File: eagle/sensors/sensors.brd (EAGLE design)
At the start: 51.7 x 35.5 mm, 4 parts

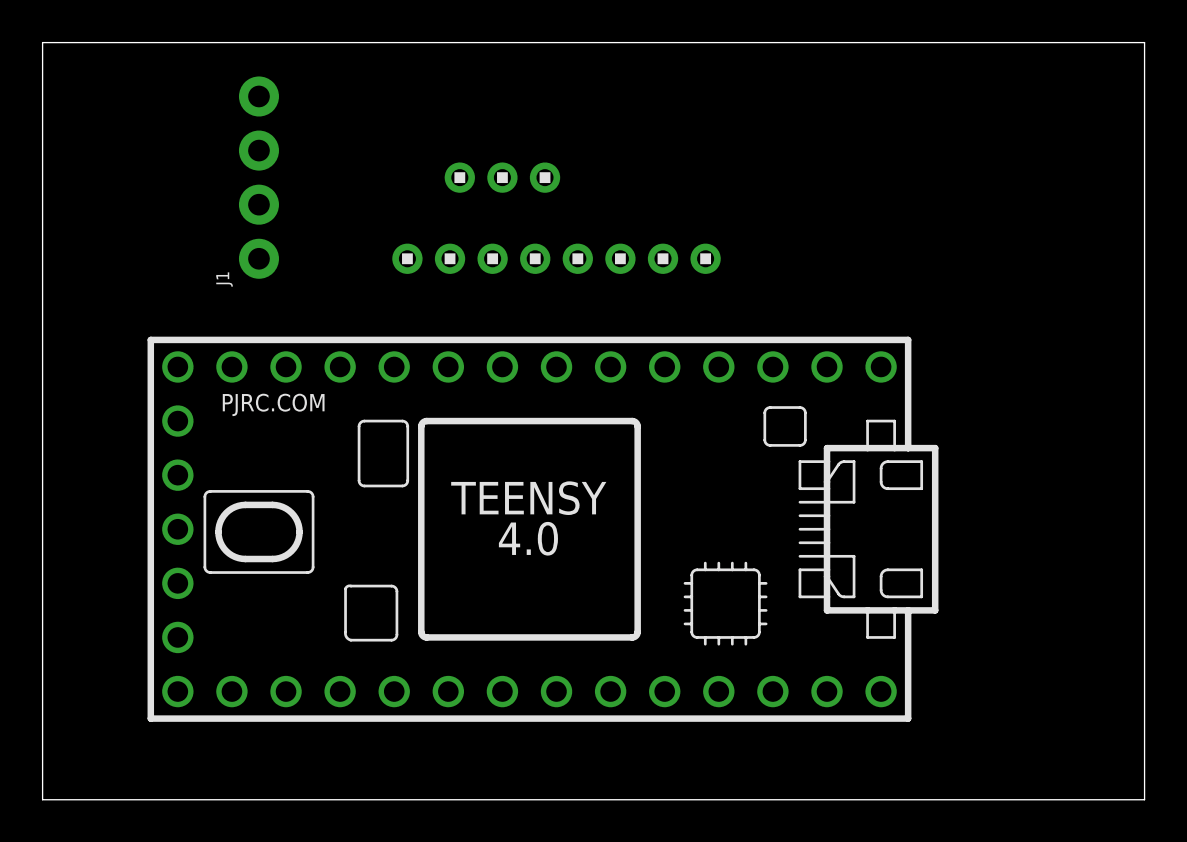
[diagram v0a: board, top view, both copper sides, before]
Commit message: new file:   eagle/sensors/sensors.brd
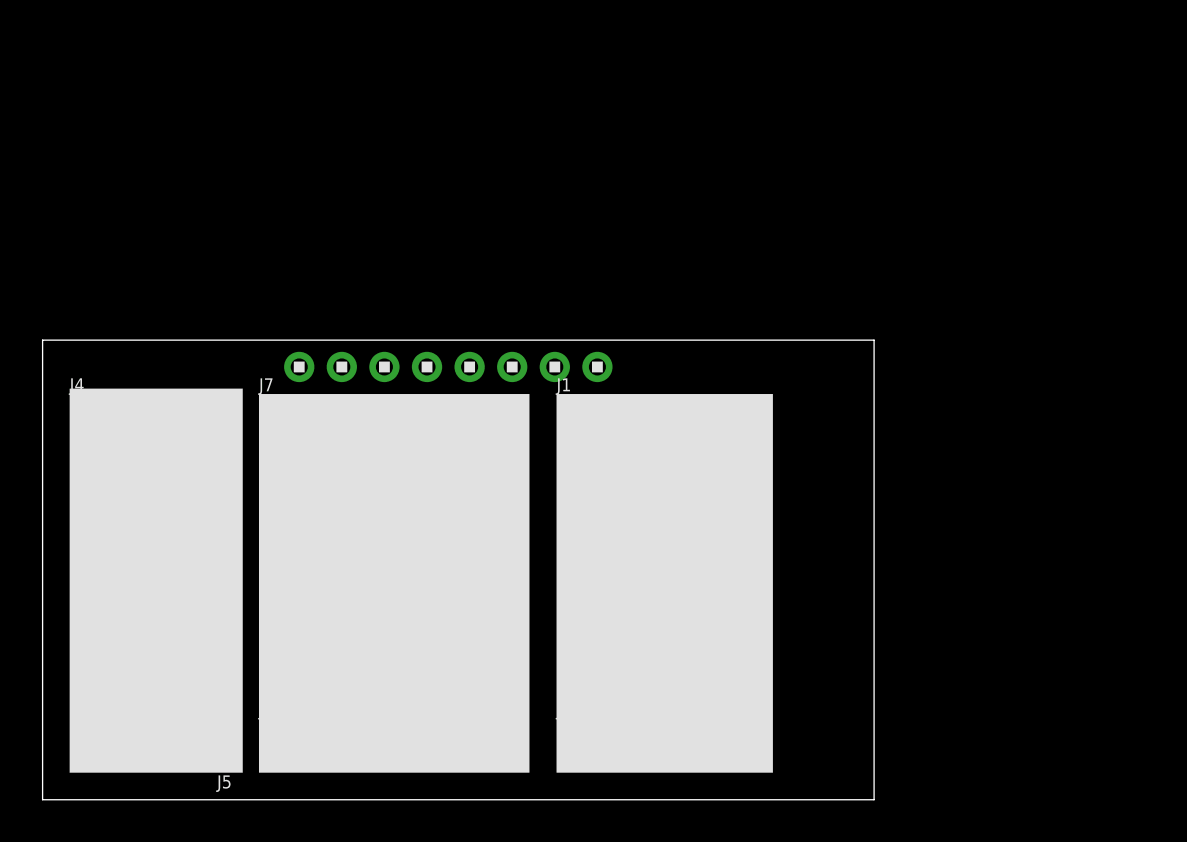
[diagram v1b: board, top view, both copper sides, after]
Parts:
- removed U$2: 1X3, headers(2mm):1X3
- removed U$3: 1X8, headers(2mm):1X8
- added J2: (no value), SparkFun-Connectors:1X04_NO_SILK
- added J3: (no value), SparkFun-Connectors:1X02_NO_SILK
- added J4, J5: (no value), SparkFun-Connectors:1X03_NO_SILK
- added J6, J7: (no value), SparkFun-Connectors:1X05_NO_SILK
- U$1: value TEENSY_4.0 -> 1X8; device TEENSY 4.0:TEENSY_4.0 -> headers(2mm):1X8
- moved J1 17.0 mm to (25.4, 17.8), turned to 0 degrees
- moved U$1 8.52 mm to (19.1, 20.3), turned to 0 degrees
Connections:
- removed net 5V: J1.4, U$2.2
- removed net SBUS: U$2.3
- removed net VBAT: J1.2
- new net EN: J2.3
- new net LED: J1.1
- new net MOT: J2.2
- new net RESET: J2.1
- new net US_INT: J6.1
- new net VL_INT: J5.3
- new net XSH: J4.3
- net 3V3: now also J3.2, J5.1, J7.4, U$1.1; no longer U$3.1
- net CS: now also J1.2, U$1.8; no longer U$3.8
- net GND: now also J3.1, J5.2, J7.5, U$1.2; no longer J1.3, U$2.1, U$3.2
- net MISO: now also J1.4, U$1.5; no longer U$3.5
- net MOSI: now also J1.3, U$1.6; no longer U$3.6
- net SCK: now also J2.4, U$1.7; no longer U$3.7
- net SCL: now also J4.2, J7.2, U$1.3; no longer U$3.3
- net SDA: now also J4.1, J7.1, U$1.4; no longer U$3.4
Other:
- board size 51.7 x 35.5 mm -> 39 x 21.6 mm
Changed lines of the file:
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@@
 <setting verticaltext="up"/>
 </settings>
-<grid distance="50" unitdist="mil" unit="mil" style="lines" multiple="1" display="no" altdistance="5" altunitdist="mil" altunit="mil"/>
+<grid distance="50" unitdist="mil" unit="mm" style="lines" multiple="1" display="no" altdistance="5" altunitdist="mil" altunit="mil"/>
 <layers>
 <layer number="1" name="Top" color="4" fill="1" visible="yes" active="yes"/>
@@
 <board>
 <plain>
-<wire x1="0" y1="0" x2="51.74" y2="0" width="0" layer="20"/>
-<wire x1="51.74" y1="0" x2="51.74" y2="35.55" width="0" layer="20"/>
-<wire x1="51.74" y1="35.55" x2="0" y2="35.55" width="0" layer="20"/>
-<wire x1="0" y1="35.55" x2="0" y2="0" width="0" layer="20"/>
+<wire x1="0" y1="0" x2="39.04" y2="0" width="0" layer="20"/>
+<wire x1="39.04" y1="0" x2="39.04" y2="21.58" width="0" layer="20"/>
+<wire x1="39.04" y1="21.58" x2="0" y2="21.58" width="0" layer="20"/>
+<wire x1="0" y1="21.58" x2="0" y2="0" width="0" layer="20"/>
+<rectangle x1="10.16" y1="1.27" x2="22.86" y2="19.05" layer="21"/>
+<rectangle x1="1.27" y1="1.27" x2="9.398" y2="19.304" layer="21" rot="R180"/>
+<rectangle x1="24.13" y1="1.27" x2="34.29" y2="19.05" layer="21"/>
 </plain>
 <attributes>
@@
 </autorouter>
 <elements>
-<element name="U$1" library="TEENSY 4.0" package="TEENSY_4.0" value="TEENSY_4.0" x="22.86" y="12.7" smashed="yes" rot="R180"/>
-<element name="J1" library="SparkFun-Connectors" package="1X04_NO_SILK" value="" x="10.16" y="25.4" smashed="yes" rot="R90">
-<attribute name="NAME" x="8.763" y="24.13" size="0.6096" layer="25" font="vector" ratio="20" rot="R90"/>
-<attribute name="PROD_ID" value="CONN-09696" x="10.16" y="25.4" size="1.778" layer="27" rot="R90" display="off"/>
-<attribute name="VALUE" x="12.192" y="24.13" size="0.6096" layer="27" font="vector" ratio="20" rot="R90"/>
-</element>
-<element name="U$2" library="headers(2mm)" package="1X3" value="1X3" x="21.59" y="29.21" smashed="yes"/>
-<element name="U$3" library="headers(2mm)" package="1X8" value="1X8" x="24.13" y="25.4" smashed="yes"/>
+<element name="U$1" library="headers(2mm)" package="1X8" value="1X8" x="19.05" y="20.32" smashed="yes"/>
+<element name="J1" library="SparkFun-Connectors" package="1X04_NO_SILK" value="" x="25.4" y="17.78" smashed="yes">
+<attribute name="NAME" x="24.13" y="19.177" size="0.6096" layer="25" font="vector" ratio="20"/>
+<attribute name="PROD_ID" value="CONN-09696" x="25.4" y="17.78" size="1.778" layer="27" display="off"/>
+<attribute name="VALUE" x="24.13" y="15.748" size="0.6096" layer="27" font="vector" ratio="20"/>
+</element>
+<element name="J2" library="SparkFun-Connectors" package="1X04_NO_SILK" value="" x="25.4" y="2.54" smashed="yes">
+<attribute name="NAME" x="24.13" y="3.937" size="0.6096" layer="25" font="vector" ratio="20"/>
+<attribute name="PROD_ID" value="CONN-09696" x="25.4" y="2.54" size="1.778" layer="27" display="off"/>
+<attribute name="VALUE" x="24.13" y="0.508" size="0.6096" layer="27" font="vector" ratio="20"/>
+</element>
+<element name="J3" library="SparkFun-Connectors" package="1X02_NO_SILK" value="" x="33.02" y="8.89" smashed="yes" rot="R90">
+<attribute name="NAME" x="31.623" y="7.62" size="0.6096" layer="25" font="vector" ratio="20" rot="R90"/>
+<attribute name="VALUE" x="35.052" y="7.62" size="0.6096" layer="27" font="vector" ratio="20" rot="R90"/>
+</element>
+<element name="J4" library="SparkFun-Connectors" package="1X03_NO_SILK" value="" x="2.54" y="17.78" smashed="yes">
+<attribute name="NAME" x="1.27" y="19.177" size="0.6096" layer="25" font="vector" ratio="20"/>
+<attribute name="VALUE" x="1.27" y="15.748" size="0.6096" layer="27" font="vector" ratio="20"/>
+</element>
+<element name="J5" library="SparkFun-Connectors" package="1X03_NO_SILK" value="" x="7.62" y="2.54" smashed="yes" rot="R180">
+<attribute name="NAME" x="8.89" y="1.143" size="0.6096" layer="25" font="vector" ratio="20" rot="R180"/>
+<attribute name="VALUE" x="8.89" y="4.572" size="0.6096" layer="27" font="vector" ratio="20" rot="R180"/>
+</element>
+<element name="J6" library="SparkFun-Connectors" package="1X05_NO_SILK" value="" x="11.43" y="2.54" smashed="yes">
+<attribute name="NAME" x="10.16" y="3.937" size="0.6096" layer="25" font="vector" ratio="20"/>
+<attribute name="VALUE" x="10.16" y="0.508" size="0.6096" layer="27" font="vector" ratio="20"/>
+</element>
+<element name="J7" library="SparkFun-Connectors" package="1X05_NO_SILK" value="" x="11.43" y="17.78" smashed="yes">
+<attribute name="NAME" x="10.16" y="19.177" size="0.6096" layer="25" font="vector" ratio="20"/>
+<attribute name="VALUE" x="10.16" y="15.748" size="0.6096" layer="27" font="vector" ratio="20"/>
+</element>
 </elements>
 <signals>
+<signal name="3V3">
+<contactref element="U$1" pad="1"/>
+<contactref element="J3" pad="2"/>
+<contactref element="J5" pad="1"/>
+<contactref element="J7" pad="4"/>
+<wire x1="19.05" y1="17.78" x2="33.02" y2="11.43" width="0" layer="19" extent="1-1"/>
+<wire x1="7.62" y1="2.54" x2="19.05" y2="17.78" width="0" layer="19" extent="1-1"/>
+<wire x1="12.05" y1="20.32" x2="7.62" y2="2.54" width="0" layer="19" extent="1-1"/>
+</signal>
 <signal name="GND">
+<contactref element="U$1" pad="2"/>
+<contactref element="J3" pad="1"/>
+<contactref element="J5" pad="2"/>
+<contactref element="J7" pad="5"/>
+<wire x1="21.59" y1="17.78" x2="33.02" y2="8.89" width="0" layer="19" extent="1-1"/>
+<wire x1="5.08" y1="2.54" x2="21.59" y2="17.78" width="0" layer="19" extent="1-1"/>
+<wire x1="14.05" y1="20.32" x2="21.59" y2="17.78" width="0" layer="19" extent="1-1"/>
+</signal>
+<signal name="SCL">
+<contactref element="U$1" pad="3"/>
+<contactref element="J4" pad="2"/>
+<contactref element="J7" pad="2"/>
+<wire x1="5.08" y1="17.78" x2="13.97" y2="17.78" width="0" layer="19" extent="1-1"/>
+<wire x1="16.05" y1="20.32" x2="5.08" y2="17.78" width="0" layer="19" extent="1-1"/>
+</signal>
+<signal name="SDA">
+<contactref element="U$1" pad="4"/>
+<contactref element="J4" pad="1"/>
+<contactref element="J7" pad="1"/>
+<wire x1="2.54" y1="17.78" x2="11.43" y2="17.78" width="0" layer="19" extent="1-1"/>
+<wire x1="18.05" y1="20.32" x2="2.54" y2="17.78" width="0" layer="19" extent="1-1"/>
+</signal>
+<signal name="MISO">
+<contactref element="U$1" pad="5"/>
+<contactref element="J1" pad="4"/>
+<wire x1="33.02" y1="17.78" x2="20.05" y2="20.32" width="0" layer="19" extent="1-1"/>
+</signal>
+<signal name="MOSI">
+<contactref element="U$1" pad="6"/>
 <contactref element="J1" pad="3"/>
-<contactref element="U$2" pad="1"/>
-<contactref element="U$3" pad="2"/>
-<wire x1="10.16" y1="30.48" x2="19.59" y2="29.21" width="0" layer="19" extent="1-1"/>
-<wire x1="19.13" y1="25.4" x2="10.16" y2="30.48" width="0" layer="19" extent="1-1"/>
-</signal>
-<signal name="5V">
-<contactref element="J1" pad="4"/>
-<contactref element="U$2" pad="2"/>
-<wire x1="21.59" y1="29.21" x2="10.16" y2="33.02" width="0" layer="19" extent="1-1"/>
-</signal>
-<signal name="VBAT">
+<wire x1="30.48" y1="17.78" x2="22.05" y2="20.32" width="0" layer="19" extent="1-1"/>
+</signal>
+<signal name="SCK">
+<contactref element="U$1" pad="7"/>
+<contactref element="J2" pad="4"/>
+<wire x1="33.02" y1="2.54" x2="24.05" y2="20.32" width="0" layer="19" extent="1-1"/>
+</signal>
+<signal name="CS">
+<contactref element="U$1" pad="8"/>
 <contactref element="J1" pad="2"/>
-</signal>
-<signal name="SBUS">
-<contactref element="U$2" pad="3"/>
-</signal>
-<signal name="3V3">
-<contactref element="U$3" pad="1"/>
-</signal>
-<signal name="SCL">
-<contactref element="U$3" pad="3"/>
-</signal>
-<signal name="SDA">
-<contactref element="U$3" pad="4"/>
-</signal>
-<signal name="MISO">
-<contactref element="U$3" pad="5"/>
-</signal>
-<signal name="MOSI">
-<contactref element="U$3" pad="6"/>
-</signal>
-<signal name="SCK">
-<contactref element="U$3" pad="7"/>
-</signal>
-<signal name="CS">
-<contactref element="U$3" pad="8"/>
+<wire x1="27.94" y1="17.78" x2="26.05" y2="20.32" width="0" layer="19" extent="1-1"/>
+</signal>
+<signal name="LED">
+<contactref element="J1" pad="1"/>
+</signal>
+<signal name="RESET">
+<contactref element="J2" pad="1"/>
+</signal>
+<signal name="MOT">
+<contactref element="J2" pad="2"/>
+</signal>
+<signal name="EN">
+<contactref element="J2" pad="3"/>
+</signal>
+<signal name="XSH">
+<contactref element="J4" pad="3"/>
+</signal>
+<signal name="VL_INT">
+<contactref element="J5" pad="3"/>
+</signal>
+<signal name="US_INT">
+<contactref element="J6" pad="1"/>
 </signal>
 </signals>
@@
 </board>
 </drawing>
-<compatibility>
-<note version="6.3" minversion="6.2.2" severity="warning">
-Since Version 6.2.2 text objects can contain more than one line,
-which will not be processed correctly with this version.
-</note>
-</compatibility>
 </eagle>
